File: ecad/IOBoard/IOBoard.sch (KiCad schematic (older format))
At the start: 11 parts, among them J1 SN37A12B, J2 PJ-102A, J3 toEffectsBoard, J4 SN37A12A, U1 FS57003PLT2B2M2QE

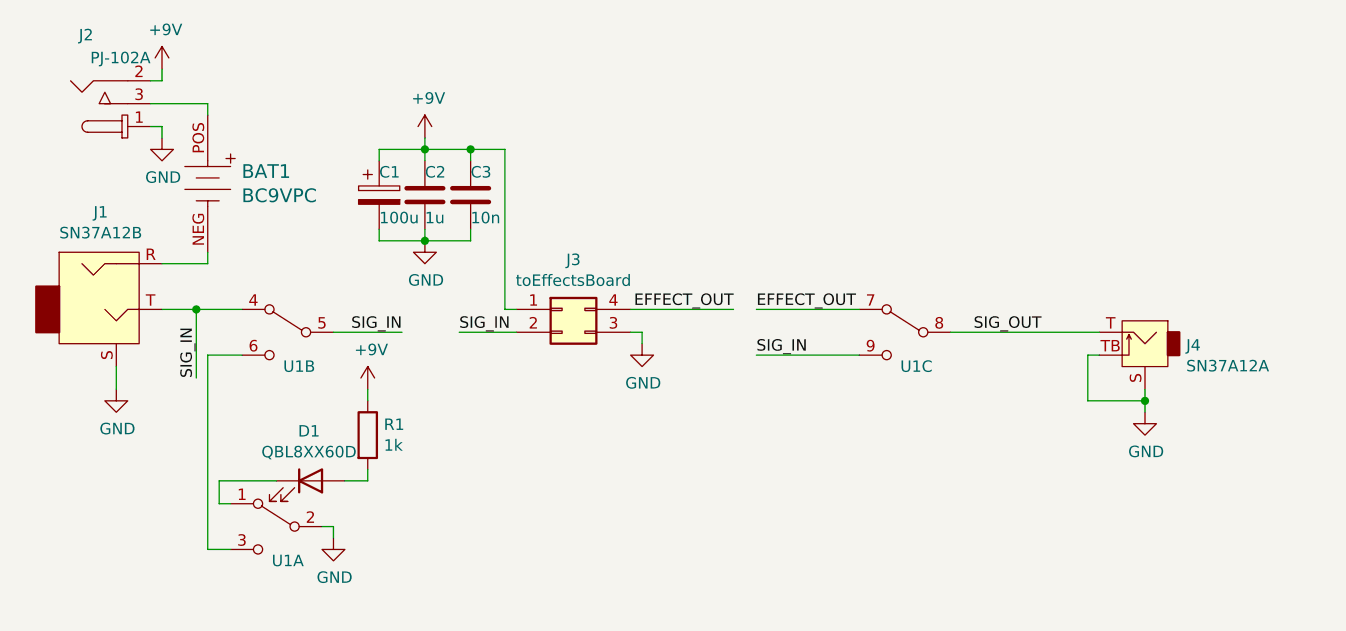
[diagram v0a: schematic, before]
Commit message: Update before switch to single-board design
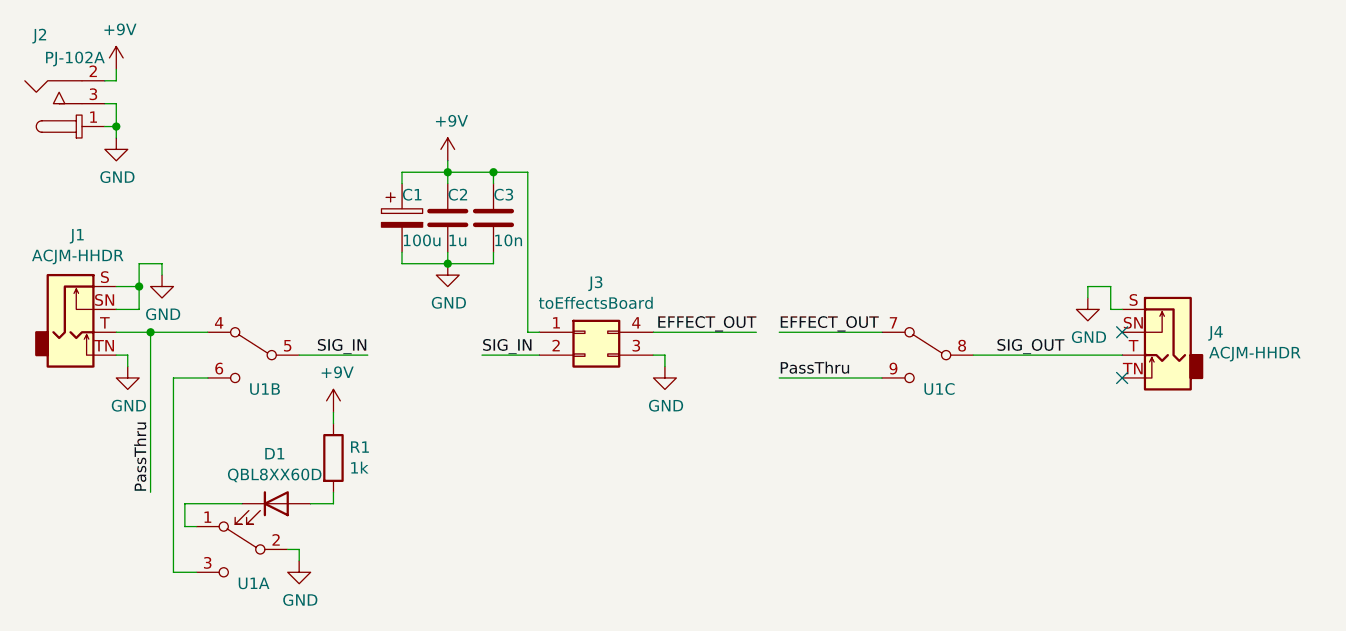
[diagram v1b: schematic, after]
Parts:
- removed BAT1: BC9VPC, DigiKey:PinHeader_1x2_P2.54mm, symbol dk_Battery-Holders-Clips-Contacts:BC9VPC
- removed J1: SN37A12B, screaming-panda:Switchcraft_SN37A12B, symbol screaming-panda:SN37A12B
- removed J4: SN37A12A, screaming-panda:Switchcraft_SN37A12A, symbol screaming-panda:SN37A12A
- added J1, J4: ACJM-HHDR, screaming-panda:ACJM-HHDR, symbol Connector:AudioJack2_Switch
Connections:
- net GND: now also J2.3, J1.S, J1.SN, J1.TN, J4.S
- net SIG_IN: no longer U1.4, U1.9
- net SIG_OUT: now also J4.T
- new net PassThru: J1.T, U1.4, U1.9
- no-connect marks 0 -> 2
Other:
- moved on the sheet: C1, C2, C3, D1, J2, J3, R1, U1A, U1B, U1C
